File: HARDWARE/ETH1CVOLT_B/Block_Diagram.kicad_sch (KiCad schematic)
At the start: 0 parts

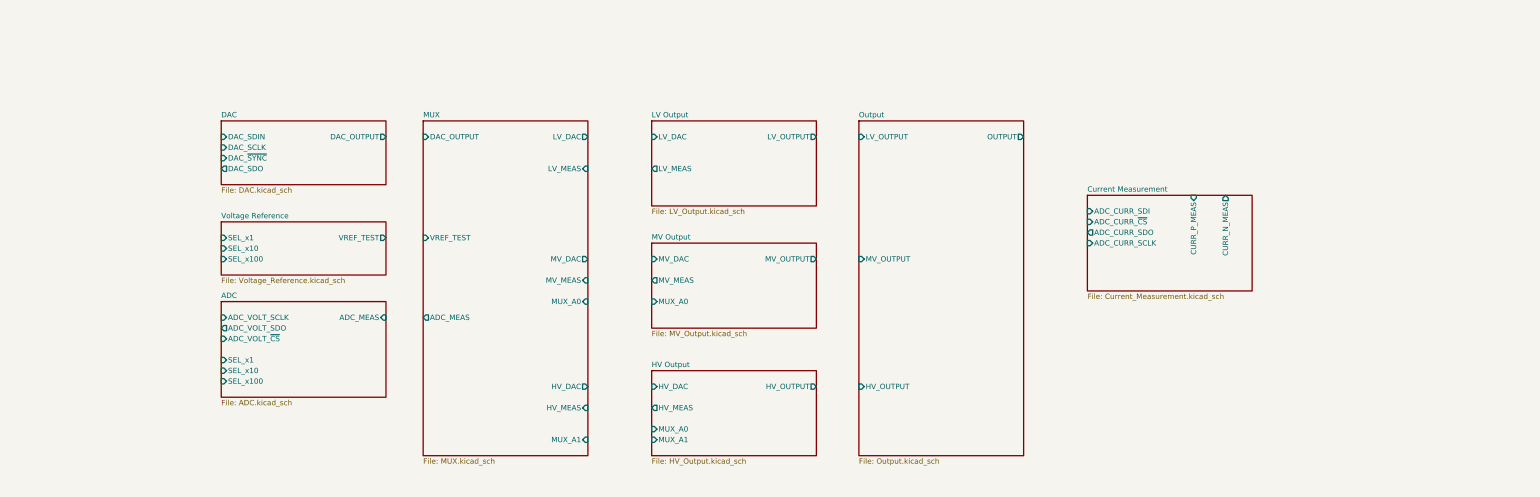
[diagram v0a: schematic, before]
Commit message: Development
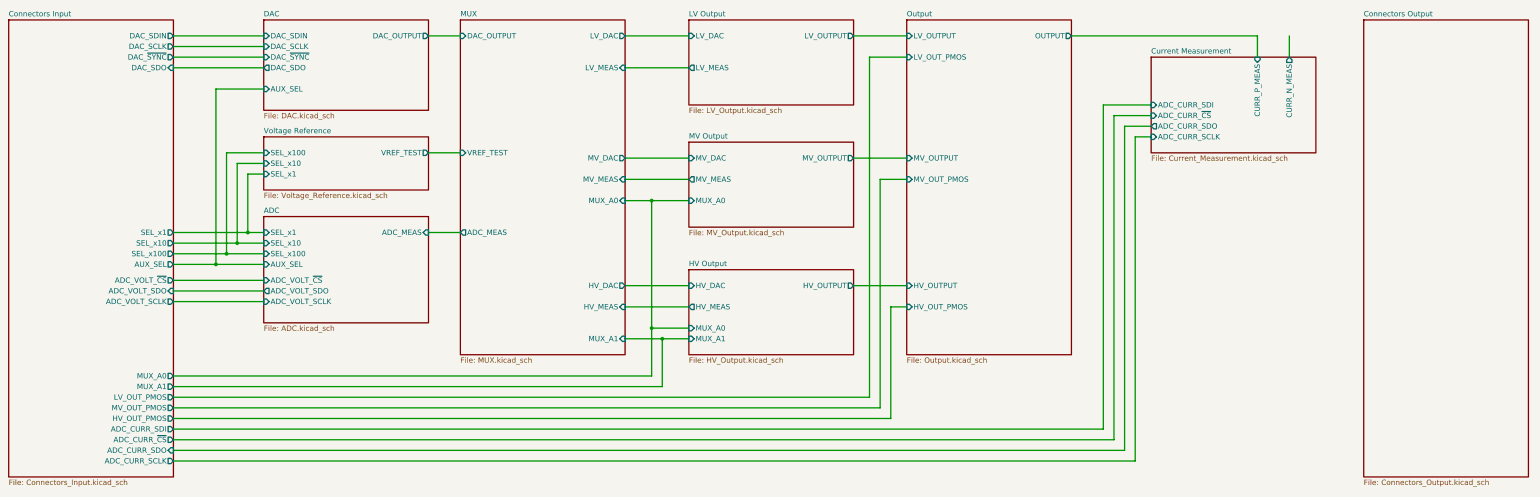
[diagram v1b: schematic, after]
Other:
- added sheet Connectors Input (Connectors_Input.kicad_sch)
- added sheet Connectors Output (Connectors_Output.kicad_sch)
- sheet ADC ports: added AUX_SEL; removed none
- sheet DAC ports: added AUX_SEL; removed none
- sheet Output ports: added HV_OUT_PMOS, LV_OUT_PMOS, MV_OUT_PMOS; removed none
